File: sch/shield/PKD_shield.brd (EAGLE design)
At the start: 68.6 x 53.3 mm, 30 parts, among them IC1 TL072P, IC2 PIC12F683P, IC3 74HCT244N, Q1 BS170

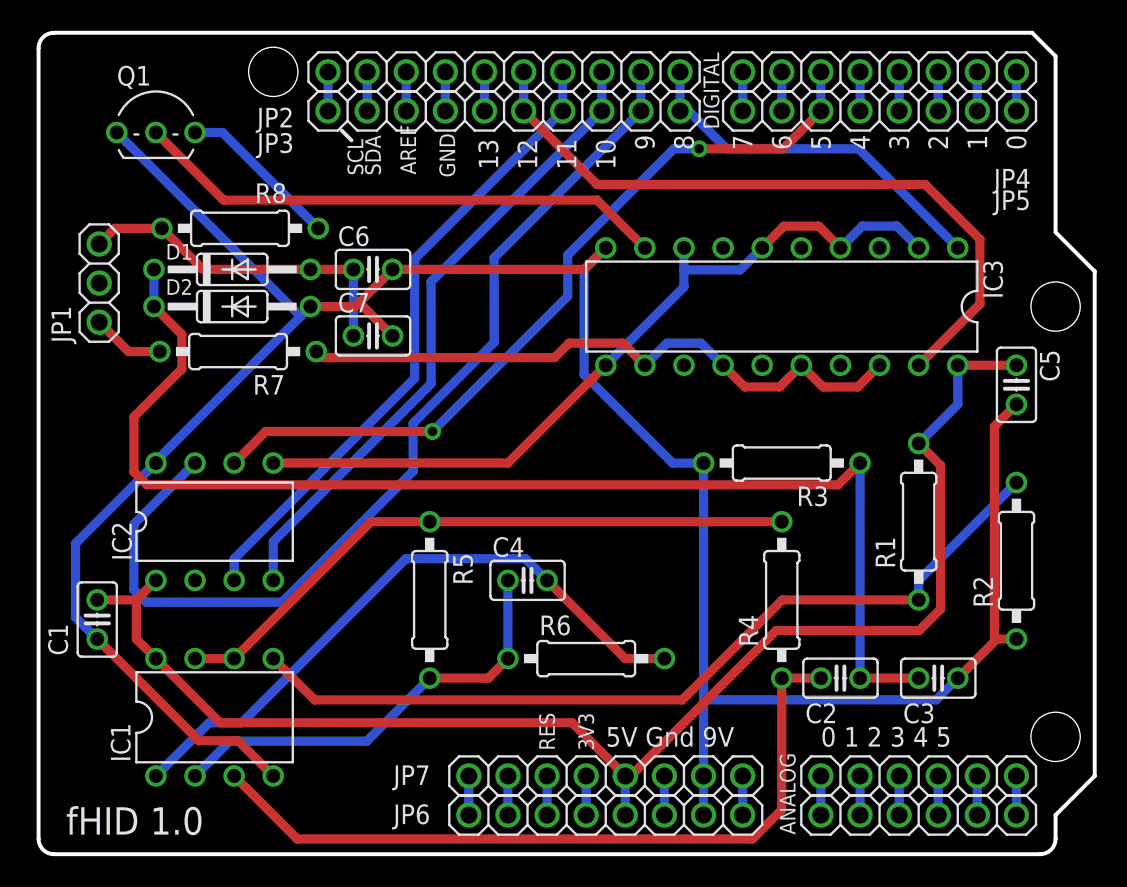
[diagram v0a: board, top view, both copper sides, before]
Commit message: New 3d model for v2.0
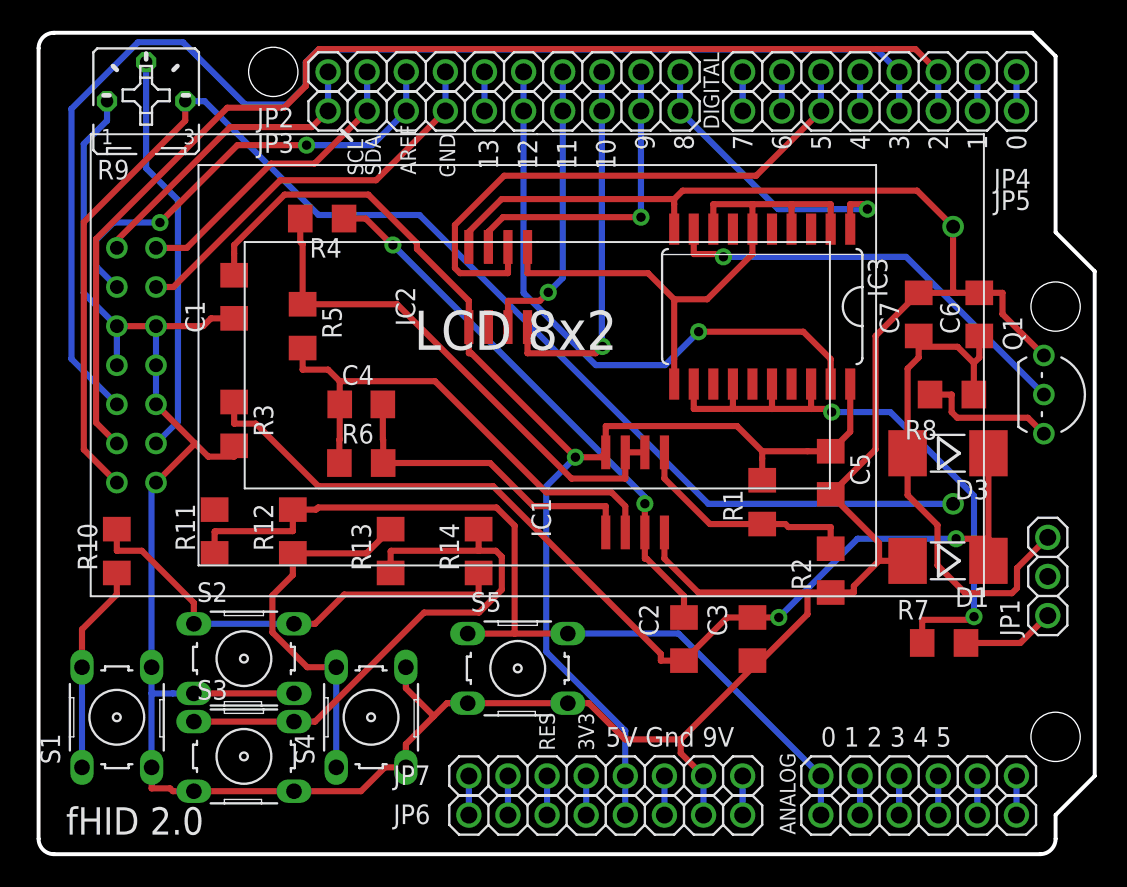
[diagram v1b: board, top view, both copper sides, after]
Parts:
- removed D2: 1N4148, diode:DO35-10
- added D3: 1N4148, diode:MELF-MLL41
- added LCD1: LCD8X2, various:LCD8X2
- added R10: 3k3, rcl:R1206
- added R11: 2k, rcl:R1206
- added R12: 330, rcl:R1206
- added R13: 620, rcl:R1206
- added R14: 1k, rcl:R1206
- added R9: (no value), pot:B25P
- added S1, S2, S3, S4, S5: (no value), switch-omron:B3F-10XX
- C1, C2, C3, C4, C5, C6, C7: device rcl:C025-025X050 -> rcl:C1206
- D1: device diode:DO35-10 -> diode:MELF-MLL41
- IC1: value TL072P -> TL072D; device linear:DIL08 -> linear:SO08
- IC2: value PIC12F683P -> PIC12F683SN; device microchip:DIL8 -> microchip:SO-08
- IC3: value 74HCT244N -> 74HCT244DW; device 74xx-eu:DIL20 -> 74xx-eu:SO20W
- R1, R2, R3, R4, R5, R6, R7, R8: device rcl:0207/10 -> rcl:R1206
- moved JP1 64.5 mm to (65.5, 18.0)
- moved Q1 60.1 mm to (65.3, 29.8), turned to 270 degrees
- moved D1 50.2 mm to (59.1, 19.1), turned to 180 degrees
- moved R7 49.6 mm to (58.8, 13.7), turned to 0 degrees
- moved R8 47.5 mm to (59.3, 29.8), turned to 0 degrees
- moved C6 39.5 mm to (61.1, 35.1), turned to 90 degrees
- moved R4 38.8 mm to (18.4, 41.3), turned to 180 degrees
- moved R3 35.7 mm to (12.7, 27.9), turned to 270 degrees
- moved C7 35.5 mm to (57.1, 35.1), turned to 90 degrees
- moved IC1 31.0 mm to (38.7, 23.5)
- moved IC2 23.9 mm to (29.8, 36.8)
- moved C1 22.8 mm to (12.7, 36.2)
- moved R5 19.6 mm to (17.1, 34.3)
- moved R6 19.4 mm to (21.0, 25.4)
- moved C4 15.7 mm to (21.0, 29.2)
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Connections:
- removed net N$12: JP4.5, JP5.5
- removed net N$13: JP4.6, JP5.6
- removed net N$141: JP2.9, JP3.9
- removed net N$142: JP2.10, JP3.10
- removed net N$222: JP2.8, JP3.8
- removed net N$24: JP2.7, JP3.7
- new net +5V: LCD1.K, LCD1.VDD, R9.E
- new net DB4: JP2.7, JP3.7, LCD1.DB4
- new net DB5: JP2.8, JP3.8, LCD1.DB5
- new net DB6: JP2.9, JP3.9, LCD1.DB6
- new net DB7: JP2.10, JP3.10, LCD1.DB7
- new net E: JP4.5, JP5.5, LCD1.E
- new net N$10: R12.1, R13.2, S4.1, S4.2
- new net N$2: LCD1.VO, R9.S
- new net N$6: R10.1, S1.1, S1.2
- new net N$7: R10.2, R14.1, S2.1, S2.2
- new net N$9: R13.1, R14.2, S3.1, S3.2
- new net RS: JP4.6, JP5.6, LCD1.RS
- net ANT_LO: now also D3.A; no longer D1.A
- net GND: now also D1.A, LCD1.A, LCD1.DB0, LCD1.DB1, LCD1.DB2, LCD1.DB3, LCD1.RW, LCD1.VSS, R9.A, S1.3, S1.4, S2.3, S2.4, S3.3, S3.4, S4.3, S4.4, S5.3, S5.4; no longer D2.A
- net N$17: now also D3.C; no longer D2.C
- net N$18: now also R11.1, R12.2, S5.1, S5.2
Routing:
- net +5V: track 0.00 -> 89.1 mm
- net E: track 0.00 -> 83.1 mm
- net RS: track 0.00 -> 77.7 mm
- net GND: track 164.0 -> 225.1 mm
- net N$18: track 2.54 -> 59.2 mm
- net R/E: track 63.9 -> 20.7 mm, vias 0 -> 1
- net N$16: track 56.0 -> 15.2 mm
- net N$9: track 0.00 -> 35.9 mm
- net N$7: track 0.00 -> 29.9 mm
- net DB5: track 0.00 -> 29.8 mm, vias 0 -> 2
- net N$2: track 0.00 -> 26.2 mm
- net DB4: track 0.00 -> 26.1 mm
- net N$10: track 0.00 -> 24.3 mm
- net BIT_IN: track 41.9 -> 19.3 mm, vias 0 -> 1
- net LO_PKD_U: track 41.6 -> 21.1 mm
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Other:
- board text added: "fHID 2.0"
- board text removed: "fHID 1.0"
